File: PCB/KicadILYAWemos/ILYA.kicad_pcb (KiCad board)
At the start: 2 copper layers, 6 parts

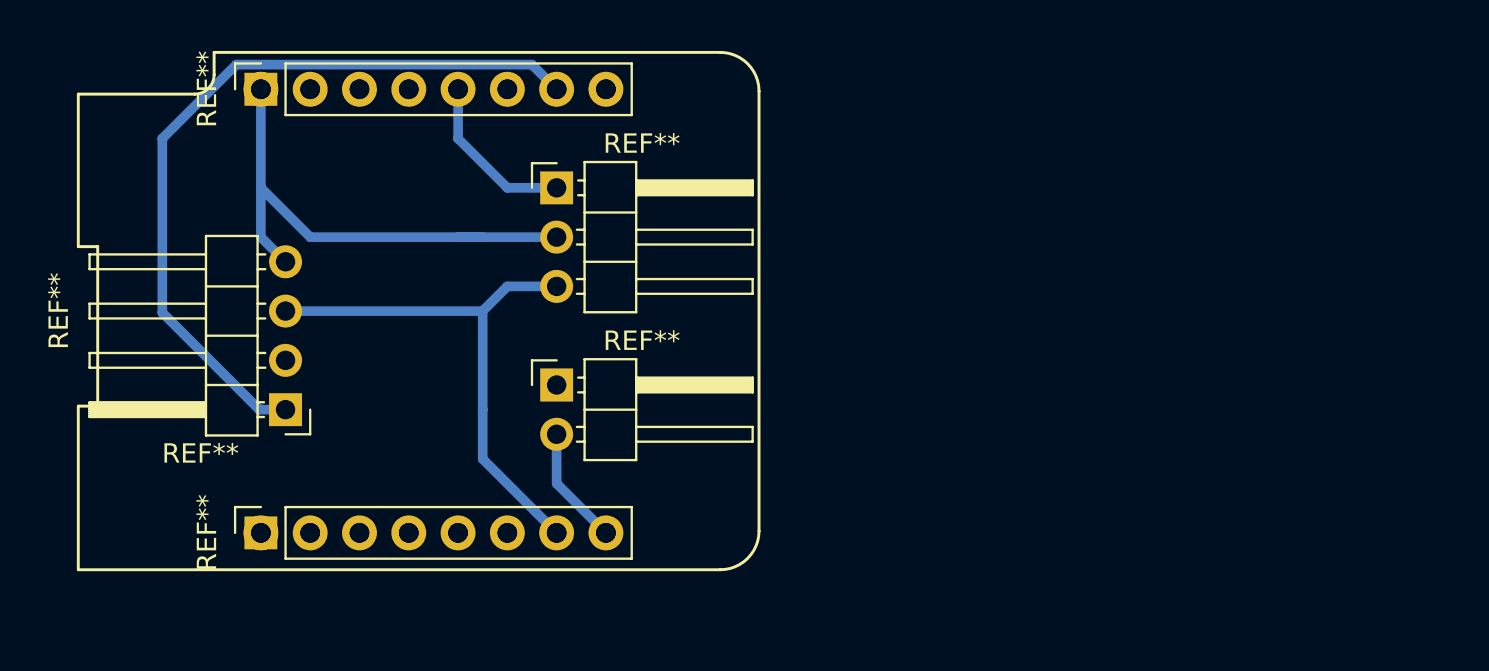
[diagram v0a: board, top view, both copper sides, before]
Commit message: PCB Wemos
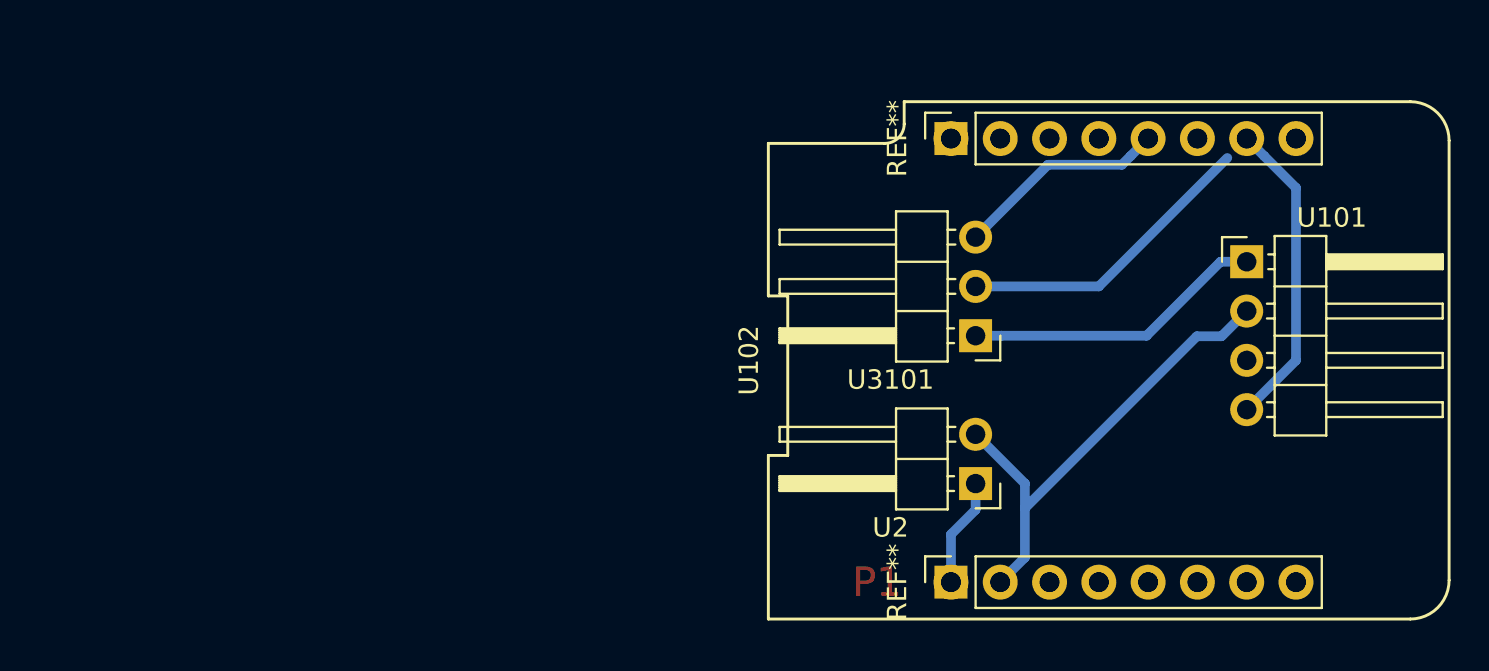
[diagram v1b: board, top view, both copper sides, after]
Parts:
- removed the REF** at (152.4, 94.0)
- removed the REF** at (158.8, 97.8)
- removed the REF** at (158.8, 87.6)
- removed the REF** at (144.8, 99.1)
- removed the REF** at (143.5, 105.4)
- removed the REF** at (143.5, 82.5)
- added REF**: PinSocket_1x08_P2.54mm_Vertical, pinSocket:PinSocket_1x08_P2.54mm_Vertical, F.Cu at (179.1, 108.0)
- added REF**: PinSocket_1x08_P2.54mm_Vertical, pinSocket:PinSocket_1x08_P2.54mm_Vertical, F.Cu at (179.1, 85.1)
- added U101: Temperature_connector, pinHeads:PinHeader_1x04_P2.54mm_Horizontal, F.Cu at (194.3, 91.4)
- added U102: WeMos_mini, wemos-d1-mini:wemos-d1-mini-with-pin-header, F.Cu at (188.0, 96.5)
- added U2: Relay_2_pins, pinHeads:PinHeader_1x02_P2.54mm_Horizontal, F.Cu at (180.3, 102.9)
- added U3101: Flow_connector, pinHeads:PinHeader_1x03_P2.54mm_Horizontal, F.Cu at (180.3, 95.2)
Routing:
- net (no net): track 109.1 -> 0.00 mm
- net GND: track 0.00 -> 40.6 mm
- net Net-(U101-Pad4): track 0.00 -> 16.1 mm
- net VCC: track 0.00 -> 15.5 mm
- net Net-(U102-Pad12): track 0.00 -> 11.0 mm
- net +5V: track 0.00 -> 5.61 mm
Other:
- board text added: "P1"
